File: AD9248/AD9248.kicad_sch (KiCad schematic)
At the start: 1 part, among them U1 AD9284BCPZ-250

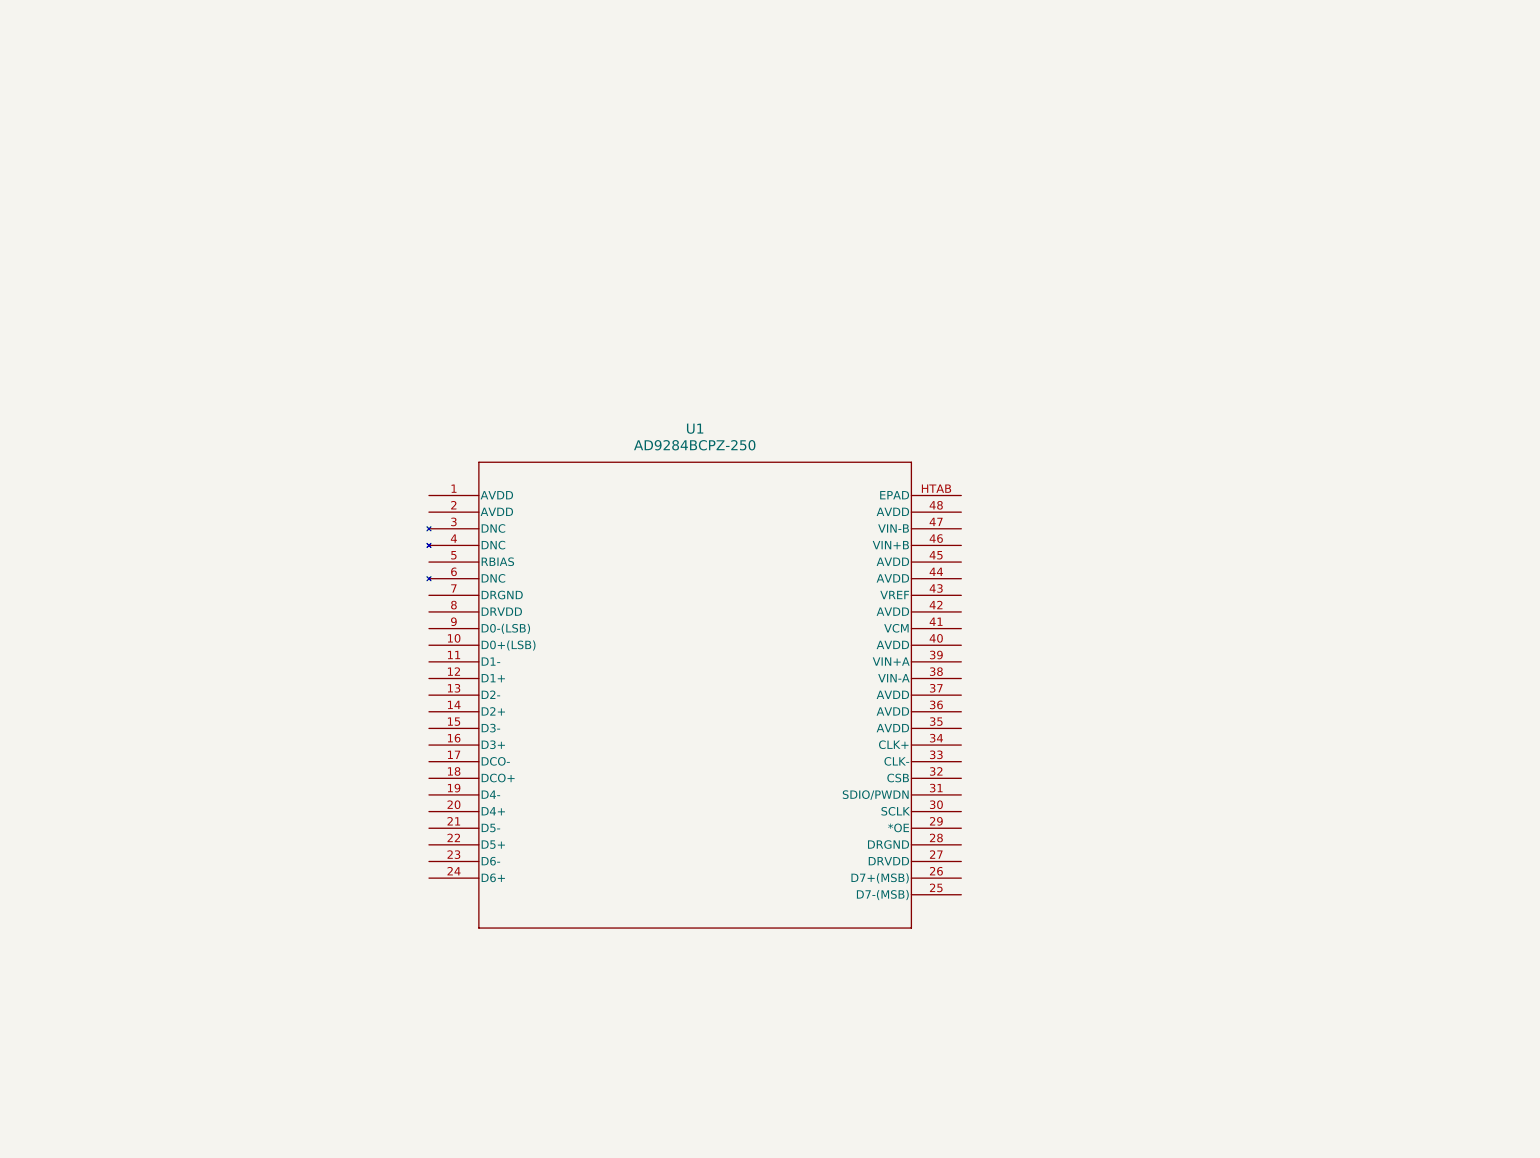
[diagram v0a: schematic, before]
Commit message: Power supply started
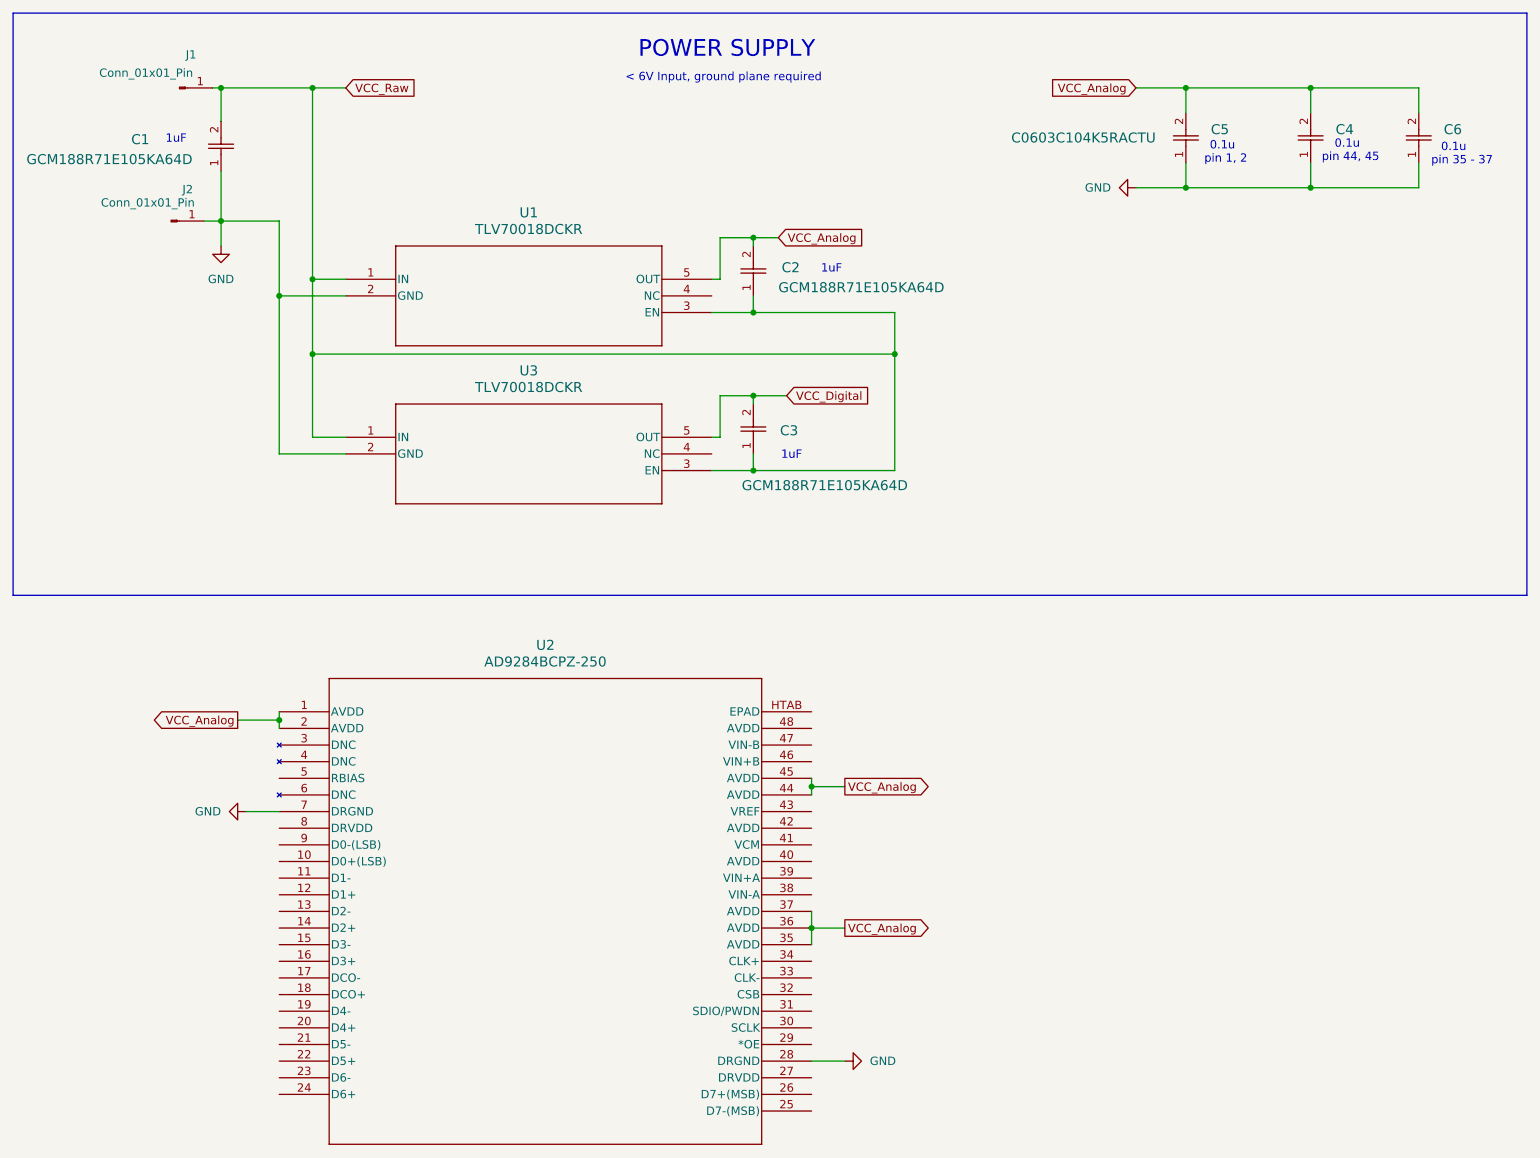
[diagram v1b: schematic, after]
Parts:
- removed U1: AD9284BCPZ-250, CP_48_12_ADI, symbol 2026-10-21_18-41-16:AD9284BCPZ-250
- added C1, C2, C3: GCM188R71E105KA64D, CAP_GCM188_MUR, symbol GCM188R71E105KA64D:GCM188R71E105KA64D
- added C4, C5, C6: C0603C104K5RACTU, CAPC17595_95N_KEM, symbol C0603C104K5RACTU:C0603C104K5RACTU
- added J1, J2: Conn_01x01_Pin, symbol Connector:Conn_01x01_Pin
- added U1, U3: TLV70018DCKR, DCK5, symbol TLV70018DCKR:TLV70018DCKR
- added U2: AD9284BCPZ-250, CP_48_12_ADI, symbol AD9248:AD9284BCPZ-250
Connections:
- new net GND: C1.1, C4.1, C5.1, C6.1, J2.1 (Pin_1), U1.2 (GND), U2.28 (DRGND), U2.7 (DRGND), U3.2 (GND)
- new net VCC_Analog: C2.2, C4.2, C5.2, C6.2, U1.5 (OUT), U2.1 (AVDD), U2.2 (AVDD), U2.35 (AVDD), U2.36 (AVDD), U2.37 (AVDD), U2.44 (AVDD), U2.45 (AVDD)
- new net VCC_Digital: C3.2, U3.5 (OUT)
- new net VCC_Raw: C1.2, C2.1, C3.1, J1.1 (Pin_1), U1.1 (IN), U1.3 (EN), U3.1 (IN), U3.3 (EN)
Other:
- note added: "0.1u"
- note added: "1uF"
- note added: "< 6V Input, ground plane required"
- note added: "POWER SUPPLY"
- note added: "pin 1, 2"
- note added: "pin 35 - 37"
- note added: "pin 44, 45"
